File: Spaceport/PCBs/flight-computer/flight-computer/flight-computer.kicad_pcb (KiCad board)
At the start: 4 copper layers, 65.1 x 48.6 mm, 107 parts, among them IC1 AP7362-33SP-13, IC2 AP7362-33SP-13, J10 5.0VOUT, J11 SWD, J12 Charge, J13 Conn_01x02, J14 Micro_SD_Card, J2 Conn_01x02, J3 Conn_01x02, J4 USB_C_Receptacle_USB2.0_16P, J5 UART, J6 UART, J7 I2C, J8 SPI, J9 3.3VOUT, U1 MS5611-01BA, U2 BMI088, U3 H3LIS331DL, U4 MMC5603NJ, U5 SAM-M10Q-00B, U6 TPS62A03DRLR, U7 STM32H723VEHx, U8 BQ25606RGER, U9 ESP32-S3-MINI-1-N4R2, Y1 ECS-2520S

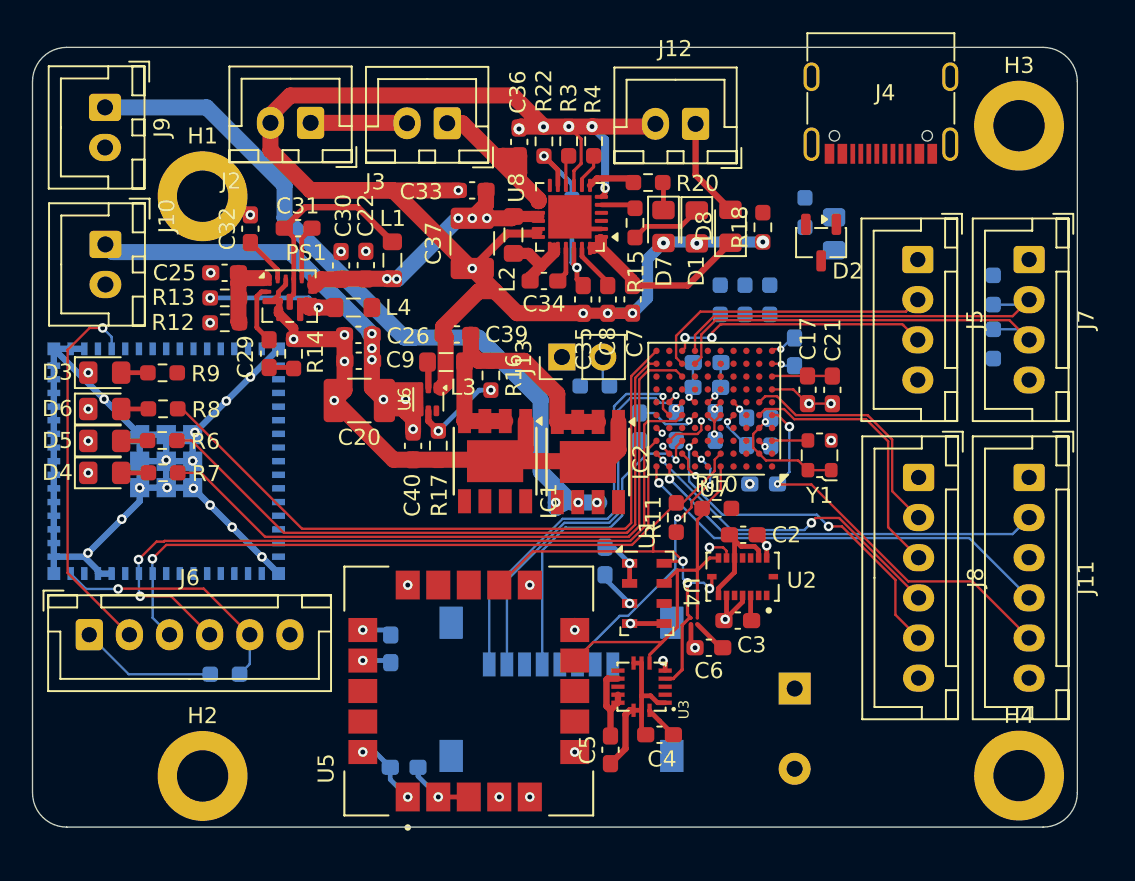
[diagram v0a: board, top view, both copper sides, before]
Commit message: PCB V1 - Needs review
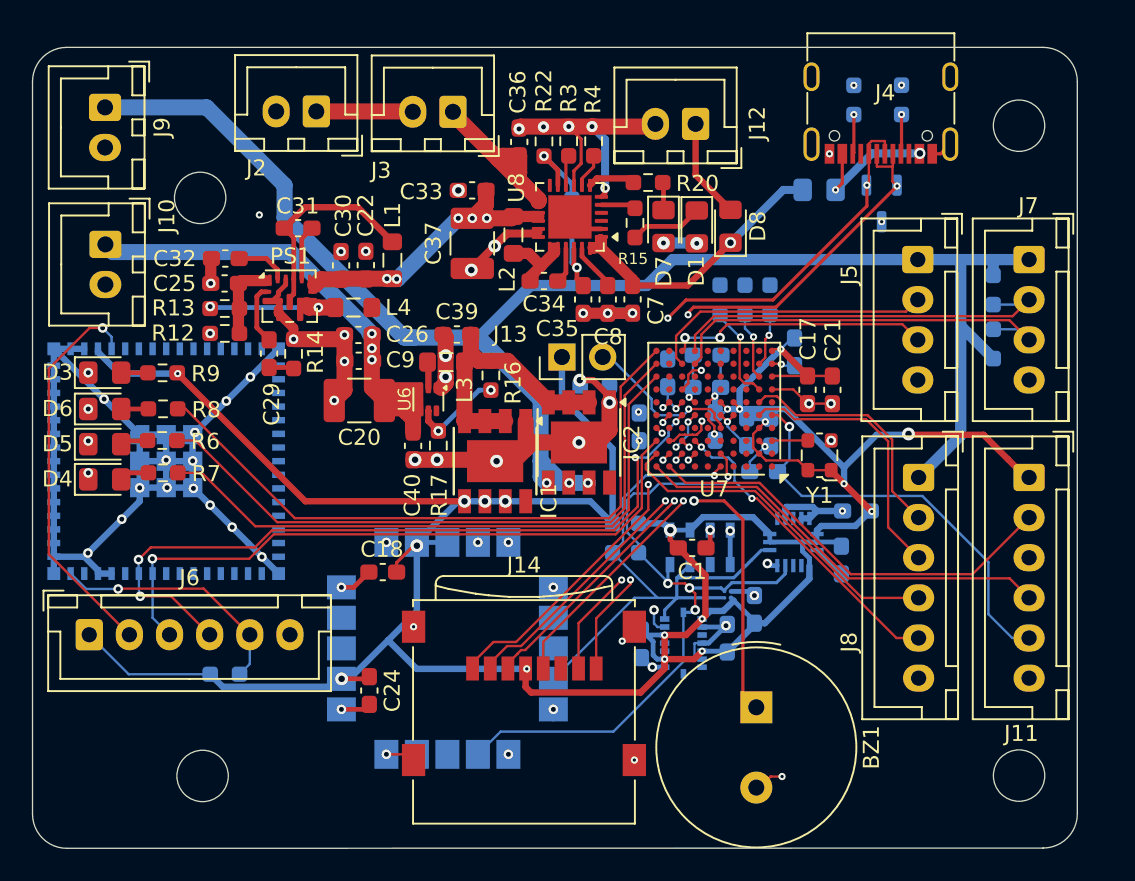
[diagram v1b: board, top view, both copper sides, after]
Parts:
- BZ1, C1, C18, C24, J14: moved to F.Cu
- C2, C3, C4, C5, C6, D2, R10, R11, R18, U1, U2, U3, U4, U5: moved to B.Cu
- H1, H2, H3, H4: footprint MountingHole:MountingHole_3.2mm_M3_DIN965_Pad -> MountingHole:MountingHole_3.2mm_M3_DIN965
- moved C5 21.4 mm to (172.7, 78.2), turned to 180 degrees
- moved C4 15.7 mm to (171.8, 81.2), turned to -90 degrees
- moved U3 13.1 mm to (168.8, 80.1), turned to 90 degrees
- moved C18 12.2 mm to (143.2, 82.0)
- moved R18 11.7 mm to (175.5, 52.5), turned to -90 degrees
- moved C2 9.29 mm to (159.3, 86.4), turned to 90 degrees
- moved R5 7.64 mm to (172.6, 52.6)
- moved R10 6.75 mm to (157.5, 79.8), turned to -90 degrees
- moved U2 5.54 mm to (161.9, 86.4), turned to 90 degrees
- moved C1 5.49 mm to (162.5, 80.5), turned to 0 degrees
- moved D2 4.49 mm to (174.3, 59.0)
- moved U1 4.38 mm to (163.0, 80.4), turned to -90 degrees
- moved C6 3.71 mm to (166.4, 84.3), turned to 90 degrees
- moved C10 3.39 mm to (161.0, 69.5), turned to 90 degrees
- moved R26 3.10 mm to (164.2, 65.0)
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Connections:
- U7 pad A2: SDMMC1_D10 -> unconnected-(U7-PC13-PadA2)
- U7 pad H10: unconnected-(U7-PB14-PadH10) -> LED3_PWM
- U7 pad H8: LED3_PWM -> unconnected-(U7-PD14-PadH8)
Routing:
- net +3V3A: track 57.6 -> 215.5 mm, vias 8 -> 20
- net GND: track 247.6 -> 181.0 mm, vias 65 -> 82
- net +3V3B: track 46.7 -> 101.5 mm
- net D+: track 0.49 -> 28.9 mm, vias 1 -> 3
- net D-: track 2.84 -> 30.4 mm, vias 1 -> 3
- net Net-(BZ1-+): track 0.00 -> 26.5 mm, vias 0 -> 2
- net SDMMC1_D2: track 0.63 -> 19.3 mm, vias 1 -> 2
- net SDMMC1_D3: track 1.74 -> 18.9 mm, vias 1 -> 2
- net I2C1_SCL: track 32.7 -> 45.2 mm, vias 3 -> 4
- net I2C1_SDA: track 26.5 -> 37.9 mm, vias 0 -> 1
- net Net-(D9-A): track 0.00 -> 8.62 mm, vias 0 -> 2
- net Net-(J13-Pin_2): track 1.98 -> 10.1 mm, vias 0 -> 1
- net SDMMC1_D1: track 25.7 -> 17.7 mm, vias 1 -> 2
- net SDMMC1_D0: track 25.2 -> 19.1 mm, vias 1 -> 2
- net Net-(U7-PA0): track 0.00 -> 6.00 mm, vias 0 -> 1
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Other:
- board size 65.1 x 48.6 mm -> 65.1 x 49.9 mm
